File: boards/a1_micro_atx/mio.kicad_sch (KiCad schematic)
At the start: 27 parts, among them J12 DE9_Plug, J13 Micro_SD_Card, U24 MAX232, U25 MIO, U26 DS1307+, X3 24MHz, Y1 32768Hz

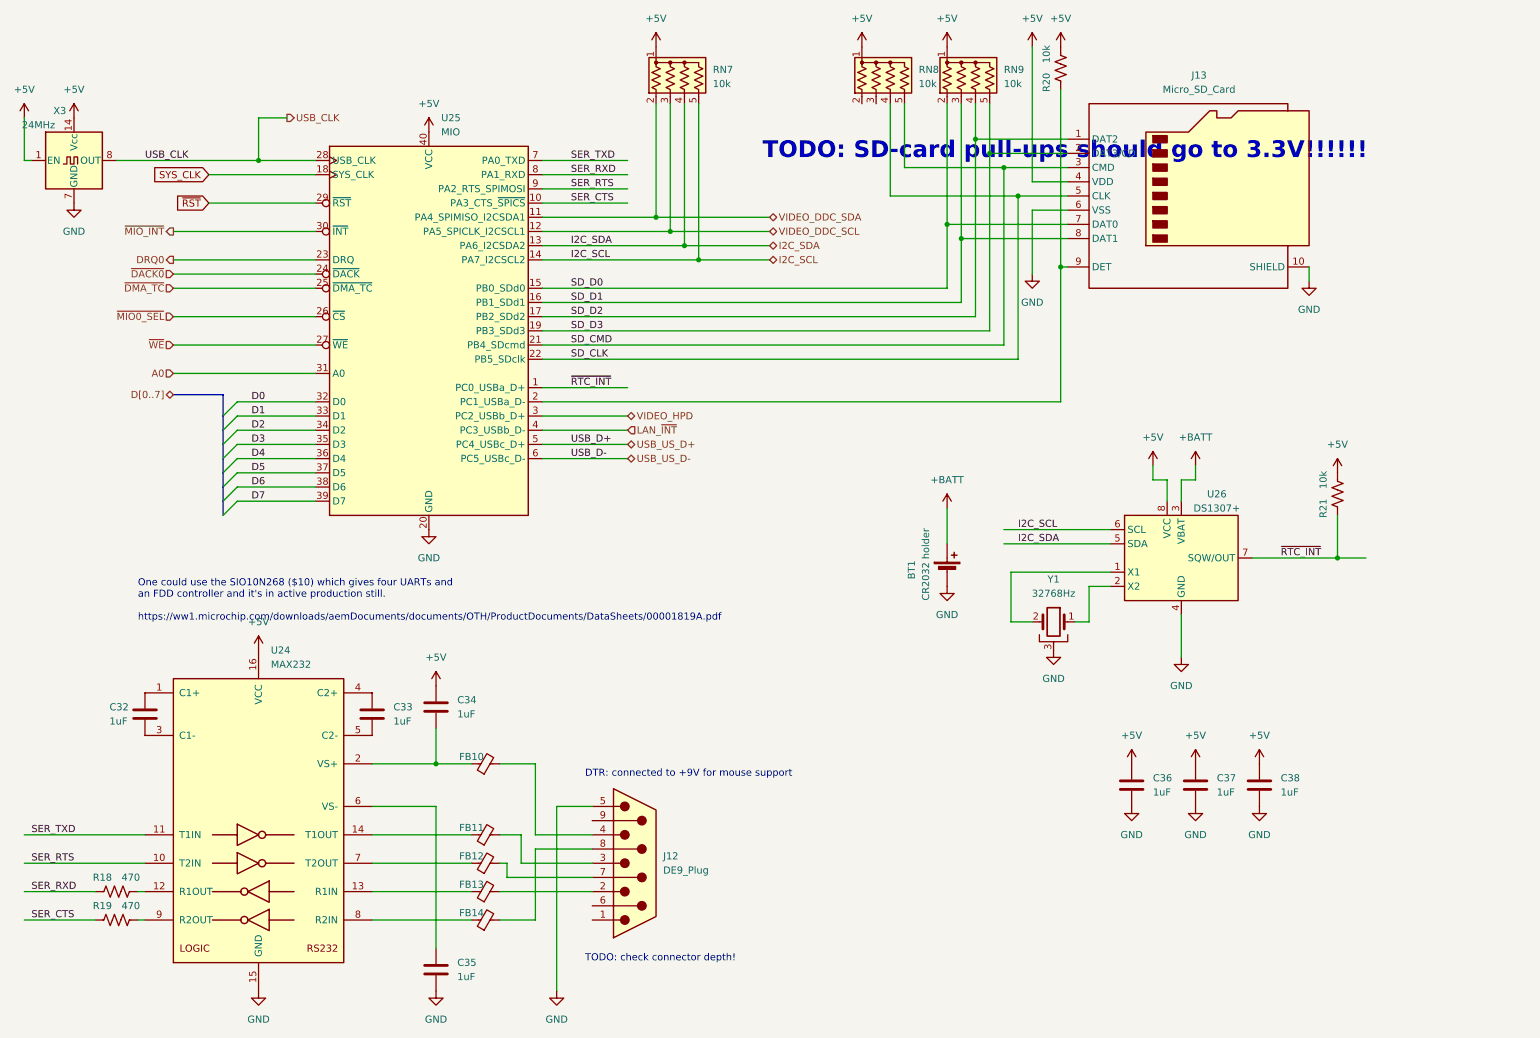
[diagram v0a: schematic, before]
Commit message: Fixed 3.3V for SDCARD; more beautification.
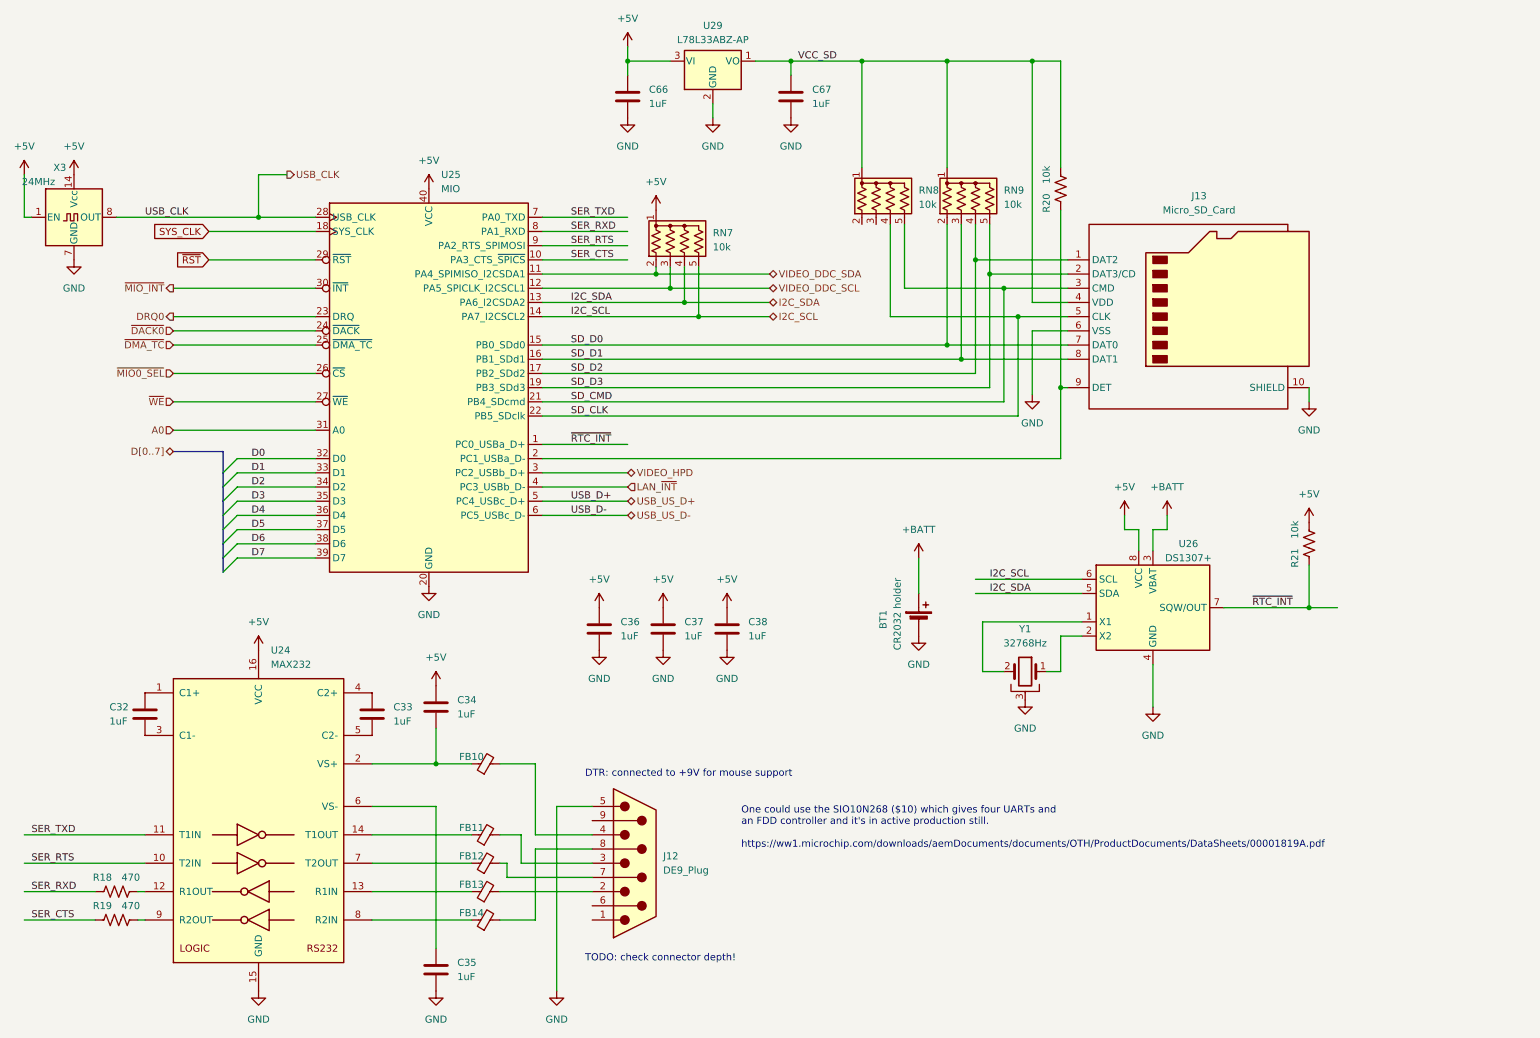
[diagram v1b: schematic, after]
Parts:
- added C66, C67: 1uF, Capacitor_THT:C_Disc_D4.7mm_W2.5mm_P5.00mm, symbol Device:C
- added U29: L78L33ABZ-AP, Package_TO_SOT_THT:TO-92_Inline, symbol Regulator_Linear:L78L05_TO92
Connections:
- net +5V: now also C66.1, U29.3 (VI); no longer J13.4 (VDD), R20.2, RN8.1 (common), RN9.1 (common)
- net GND: now also C66.2, C67.2, U29.2 (GND)
- new net VCC_SD: C67.1, J13.4 (VDD), R20.2, RN8.1 (common), RN9.1 (common), U29.1 (VO)
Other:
- note removed: "TODO: SD-card pull-ups should go to 3.3V!!!!!!"
- company: (none) -> Modular Circuits
- title: Anachron Main I/O Interfaces -> Anachron uATX Main I/O Interfaces
- moved on the sheet: BT1, C36, C37, C38, J13, R20, R21, RN7, RN8, RN9, U25, U26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
